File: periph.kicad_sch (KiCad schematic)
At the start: 25 parts, among them J4 Conn_02x08_Odd_Even, J5 Conn_02x08_Odd_Even, Q1 Q_NMOS_GSD, SW3 SLLB120200, U13 MQ-6, U14 BME680, U15 LSM6DS3, U19 PCF8574RGTR

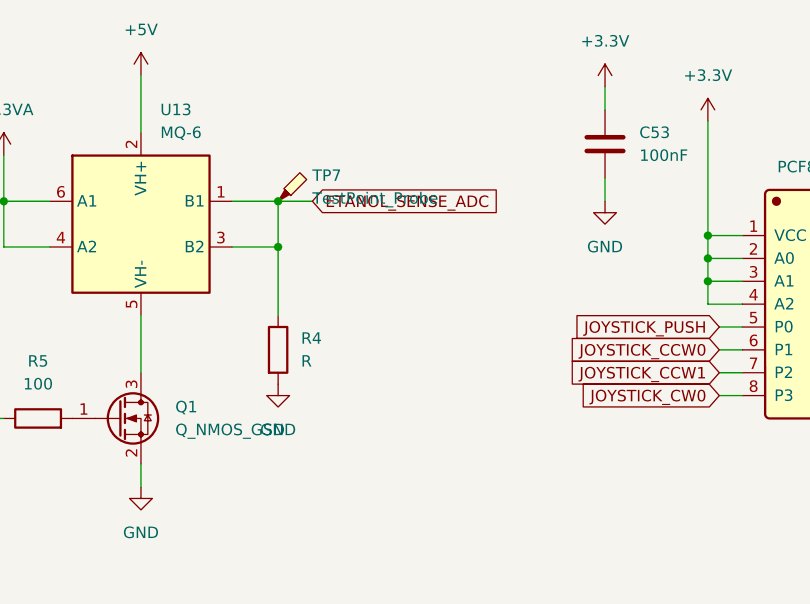
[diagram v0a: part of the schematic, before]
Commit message: Start routing
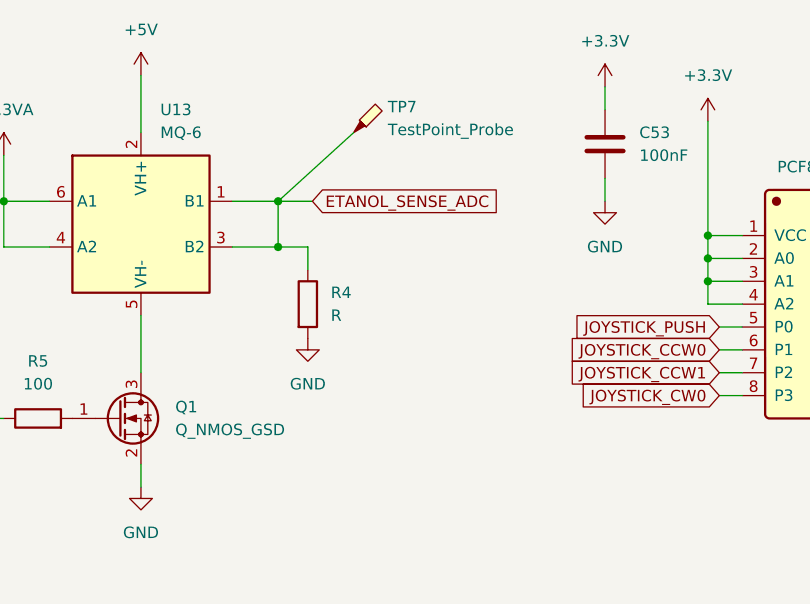
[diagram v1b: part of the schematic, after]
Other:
- moved on the sheet: R4, TP7
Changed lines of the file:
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@@
 	(wire
 		(pts
-			(xy 173.228 48.26) (xy 173.228 40.64)
+			(xy 176.53 43.18) (xy 176.53 40.64)
 		)
 		(stroke
@@
 	(wire
 		(pts
+			(xy 176.53 40.64) (xy 173.228 40.64)
+		)
+		(stroke
+			(width 0)
+			(type default)
+		)
+	)
+	(wire
+		(pts
 			(xy 109.22 143.51) (xy 119.38 143.51)
 		)
@@
 	(wire
 		(pts
+			(xy 181.61 27.94) (xy 173.228 35.56)
+		)
+		(stroke
+			(width 0)
+			(type default)
+		)
+	)
+	(wire
+		(pts
 			(xy 45.72 110.49) (xy 45.72 113.03)
 		)
@@
 	(symbol
 		(lib_id "Connector:TestPoint_Probe")
-		(at 173.228 35.56 0)
+		(at 181.61 27.94 0)
 		(unit 1)
 		(body_style 1)
@@
 		(fields_autoplaced yes)
 		(property "Reference" "TP7"
-			(at 177.038 32.7024 0)
+			(at 185.42 25.0824 0)
 			(show_name no)
 			(do_not_autoplace no)
@@
 		)
 		(property "Value" "TestPoint_Probe"
-			(at 177.038 35.2424 0)
+			(at 185.42 27.6224 0)
 			(show_name no)
 			(do_not_autoplace no)
@@
 		)
 		(property "Footprint" "TestPoint:TestPoint_THTPad_D2.0mm_Drill1.0mm"
-			(at 178.308 35.56 0)
+			(at 186.69 27.94 0)
 			(hide yes)
 			(show_name no)
@@
 		)
 		(property "Datasheet" ""
-			(at 178.308 35.56 0)
+			(at 186.69 27.94 0)
 			(hide yes)
 			(show_name no)
@@
 		)
 		(property "Description" "test point (alternative probe-style design)"
-			(at 173.228 35.56 0)
+			(at 181.61 27.94 0)
 			(hide yes)
 			(show_name no)
@@
 	(symbol
 		(lib_id "power:GND")
-		(at 173.228 55.88 0)
+		(at 176.53 50.8 0)
 		(unit 1)
 		(body_style 1)
@@
 		(fields_autoplaced yes)
 		(property "Reference" "#PWR071"
-			(at 173.228 62.23 0)
+			(at 176.53 57.15 0)
 			(hide yes)
 			(show_name no)
@@
 		)
 		(property "Value" "GND"
-			(at 173.228 60.96 0)
+			(at 176.53 55.88 0)
 			(show_name no)
 			(do_not_autoplace no)
@@
 		)
 		(property "Footprint" ""
-			(at 173.228 55.88 0)
+			(at 176.53 50.8 0)
 			(hide yes)
 			(show_name no)
@@
 		)
 		(property "Datasheet" ""
-			(at 173.228 55.88 0)
+			(at 176.53 50.8 0)
 			(hide yes)
 			(show_name no)
@@
 		)
 		(property "Description" "Power symbol creates a global label with name \"GND\" , ground"
-			(at 173.228 55.88 0)
+			(at 176.53 50.8 0)
 			(hide yes)
 			(show_name no)
@@
 	(symbol
 		(lib_id "Device:R")
-		(at 173.228 52.07 0)
+		(at 176.53 46.99 0)
 		(unit 1)
 		(body_style 1)
@@
 		(fields_autoplaced yes)
 		(property "Reference" "R4"
-			(at 175.768 50.7999 0)
+			(at 179.07 45.7199 0)
 			(show_name no)
 			(do_not_autoplace no)
@@
 		)
 		(property "Value" "R"
-			(at 175.768 53.3399 0)
+			(at 179.07 48.2599 0)
 			(show_name no)
 			(do_not_autoplace no)
@@
 		)
 		(property "Footprint" "Resistor_SMD:R_0805_2012Metric"
-			(at 171.45 52.07 90)
+			(at 174.752 46.99 90)
 			(hide yes)
 			(show_name no)
@@
 		)
 		(property "Datasheet" ""
-			(at 173.228 52.07 0)
+			(at 176.53 46.99 0)
 			(hide yes)
 			(show_name no)
@@
 		)
 		(property "Description" "Resistor"
-			(at 173.228 52.07 0)
+			(at 176.53 46.99 0)
 			(hide yes)
 			(show_name no)

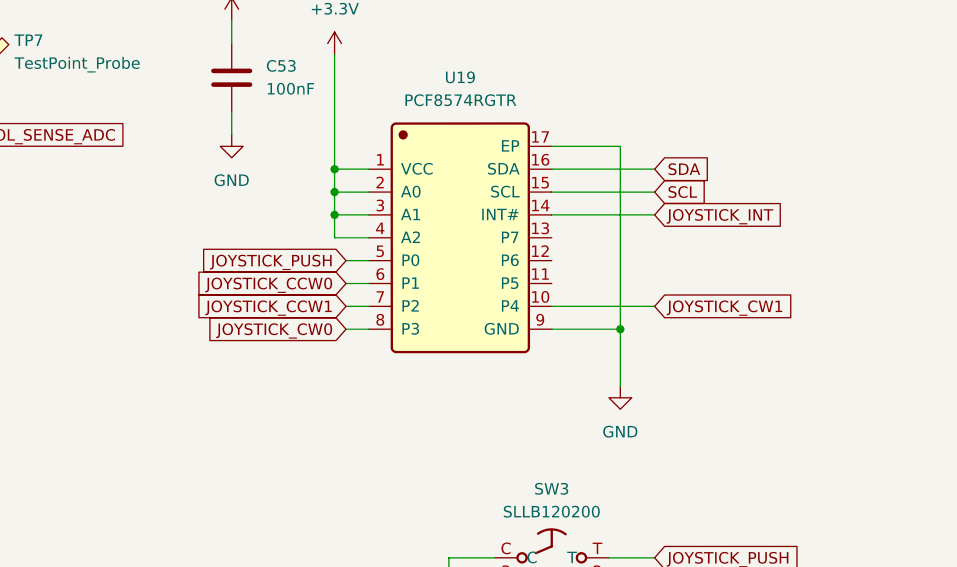
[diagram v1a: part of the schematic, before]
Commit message: Route some
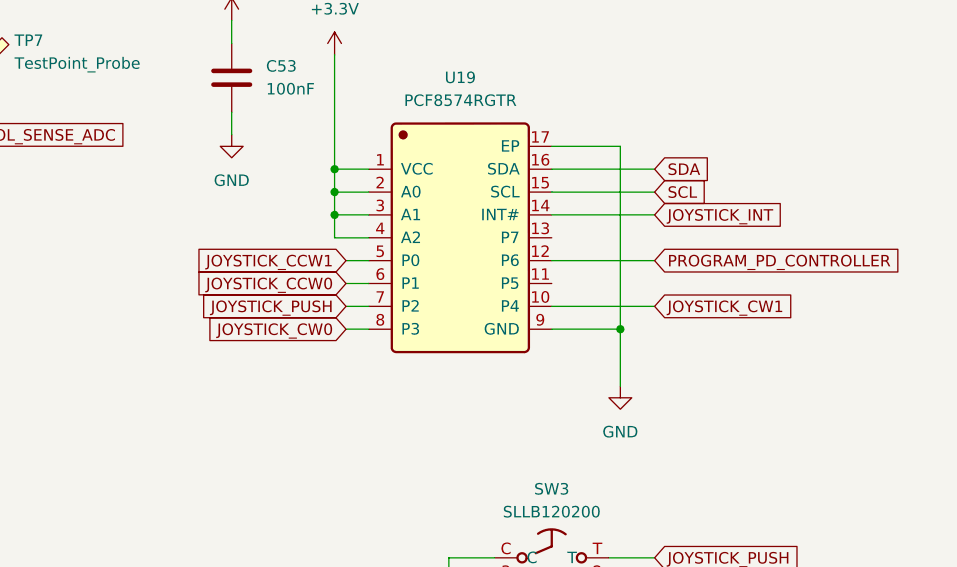
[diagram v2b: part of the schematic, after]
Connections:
- net JOYSTICK_CCW1: now also U19.5 (P0); no longer U19.7 (P2)
- net JOYSTICK_PUSH: now also U19.7 (P2); no longer U19.5 (P0)
- net PROGRAM_PD_CONTROLLER: now reaches U19.12 (P6)
